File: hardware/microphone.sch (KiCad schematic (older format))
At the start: 9 parts, among them U3 SPH0645LM4H-B

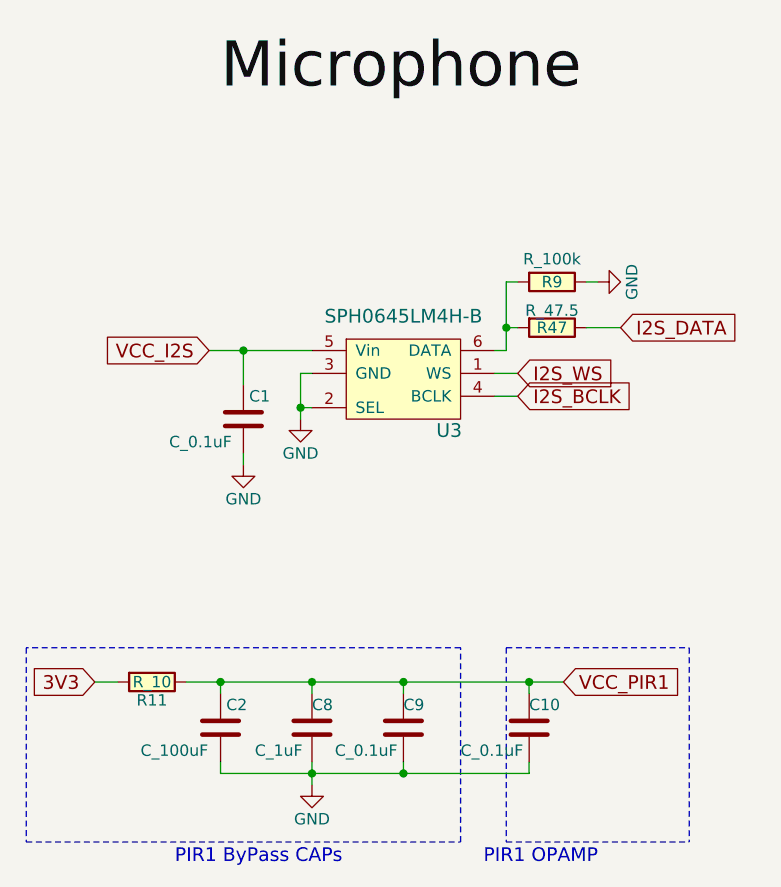
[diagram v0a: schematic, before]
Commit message: update
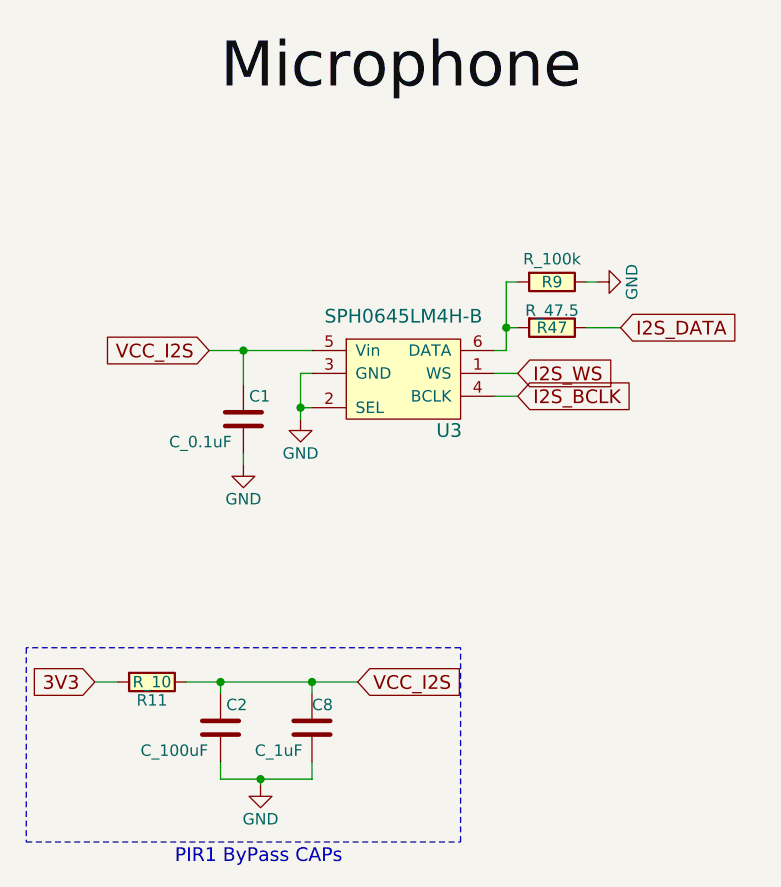
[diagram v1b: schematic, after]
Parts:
- removed C10, C9: C_0.1uF, Capacitors_SMD:C_0603, symbol C_0.1uF
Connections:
- net VCC_PIR1 is gone; now on net VCC_I2S: C2.1, C8.1, R11.1
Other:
- note removed: "PIR1 OPAMP"
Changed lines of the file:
@@
 $EndComp
 $Comp
-L GND #PWR04
+L GND #PWR08
 U 1 1 59AB3AE9
 P 4850 2350
-F 0 "#PWR04" H 4850 2100 50  0001 C CNN
+F 0 "#PWR08" H 4850 2100 50  0001 C CNN
 F 1 "GND" H 4850 2200 50  0000 C CNN
 F 2 "" H 4850 2350 50  0000 C CNN
@@
 	1    0    0    -1
 $EndComp
-Text GLabel 4450 2050 0    60   Input ~ 0
-VCC_I2S
 Text GLabel 5800 2250 2    60   Input ~ 0
 I2S_BCLK
 Text GLabel 6250 1950 2    60   Input ~ 0
 I2S_DATA
-Wire Wire Line
-	5700 2250 5800 2250
-Wire Wire Line
-	5800 2150 5700 2150
-Wire Wire Line
-	4900 2300 4850 2300
-Wire Wire Line
-	4850 2150 4850 2350
-Wire Wire Line
-	4900 2150 4850 2150
-Connection ~ 4850 2300
 Text GLabel 5800 2150 2    60   Input ~ 0
 I2S_WS
-Wire Wire Line
-	4450 2050 4900 2050
 $Comp
 L C_0.1uF C1
@@
 	1    0    0    -1
 $EndComp
-Wire Wire Line
-	4600 2200 4600 2050
-Connection ~ 4600 2050
 $Comp
-L GND #PWR05
+L GND #PWR09
 U 1 1 59B9AD4C
 P 4600 2550
-F 0 "#PWR05" H 4600 2300 50  0001 C CNN
+F 0 "#PWR09" H 4600 2300 50  0001 C CNN
 F 1 "GND" H 4600 2400 50  0000 C CNN
 F 2 "" H 4600 2550 50  0000 C CNN
@@
 	1    0    0    -1
 $EndComp
-Wire Wire Line
-	4600 2500 4600 2550
-Wire Wire Line
-	6100 1950 6250 1950
-Text GLabel 6000 3500 2    60   Input ~ 0
-VCC_PIR1
 $Comp
 L R_10 R11
@@
 $EndComp
 $Comp
-L C_0.1uF C9
-U 1 1 59B80155
-P 5300 3700
-F 0 "C9" H 5300 3800 50  0000 L CNN
-F 1 "C_0.1uF" H 5000 3600 50  0000 L CNN
-F 2 "Capacitors_SMD:C_0603" H 5400 4000 50  0001 C CNN
-F 3 "https://www.digikey.com/product-detail/en/kemet/C0603C104K5RACTU/399-5089-1-ND/1465623" H 5300 3450 50  0001 C CNN
-F 4 "C0603C104K5RACTU" H 5425 3900 60  0001 C CNN "Part Number"
-	1    5300 3700
-	1    0    0    -1
-$EndComp
-$Comp
 L C_100uF C2
 U 1 1 59B80156
@@
 $EndComp
 $Comp
-L GND #PWR06
+L GND #PWR010
 U 1 1 59B80157
-P 4900 3950
-F 0 "#PWR06" H 4900 3700 50  0001 C CNN
-F 1 "GND" H 4900 3800 50  0000 C CNN
-F 2 "" H 4900 3950 50  0000 C CNN
-F 3 "" H 4900 3950 50  0000 C CNN
-	1    4900 3950
+P 4675 3950
+F 0 "#PWR010" H 4675 3700 50  0001 C CNN
+F 1 "GND" H 4675 3800 50  0000 C CNN
+F 2 "" H 4675 3950 50  0000 C CNN
+F 3 "" H 4675 3950 50  0000 C CNN
+	1    4675 3950
 	1    0    0    -1
 $EndComp
 Text GLabel 3950 3500 0    60   Input ~ 0
 3V3
-$Comp
-L C_0.1uF C10
-U 1 1 59B80158
-P 5850 3700
-F 0 "C10" H 5850 3800 50  0000 L CNN
-F 1 "C_0.1uF" H 5550 3600 50  0000 L CNN
-F 2 "Capacitors_SMD:C_0603" H 5950 4000 50  0001 C CNN
-F 3 "https://www.digikey.com/product-detail/en/kemet/C0603C104K5RACTU/399-5089-1-ND/1465623" H 5850 3450 50  0001 C CNN
-F 4 "C0603C104K5RACTU" H 5975 3900 60  0001 C CNN "Part Number"
-	1    5850 3700
-	1    0    0    -1
-$EndComp
 Text Notes 4300 4300 0    60   ~ 0
 PIR1 ByPass CAPs
-Text Notes 5650 4300 0    60   ~ 0
-PIR1 OPAMP
-Wire Wire Line
-	4500 3850 4500 3900
-Wire Wire Line
-	4500 3900 5850 3900
-Wire Wire Line
-	5300 3900 5300 3850
-Wire Wire Line
-	4900 3850 4900 3950
-Connection ~ 4900 3900
-Wire Wire Line
-	4350 3500 6000 3500
-Wire Wire Line
-	5300 3550 5300 3500
-Connection ~ 5300 3500
-Wire Wire Line
-	4900 3550 4900 3500
-Connection ~ 4900 3500
-Wire Wire Line
-	4500 3550 4500 3500
-Connection ~ 4500 3500
-Wire Wire Line
-	3950 3500 4050 3500
-Wire Wire Line
-	5850 3550 5850 3500
-Connection ~ 5850 3500
-Wire Wire Line
-	5850 3900 5850 3850
-Connection ~ 5300 3900
-Wire Notes Line
-	3650 4200 5550 4200
-Wire Notes Line
-	5550 4200 5550 3350
-Wire Notes Line
-	5550 3350 3650 3350
-Wire Notes Line
-	5750 3350 5750 4200
-Wire Notes Line
-	5750 4200 6550 4200
-Wire Notes Line
-	5750 3350 6550 3350
-Wire Notes Line
-	3650 3350 3650 4200
-Wire Notes Line
-	6550 3350 6550 4200
 $Comp
 L R_47.5 R47
@@
 $EndComp
 $Comp
-L GND #PWR07
+L GND #PWR011
 U 1 1 59B820C6
 P 6150 1750
-F 0 "#PWR07" H 6150 1500 50  0001 C CNN
+F 0 "#PWR011" H 6150 1500 50  0001 C CNN
 F 1 "GND" H 6150 1600 50  0000 C CNN
 F 2 "" H 6150 1750 50  0000 C CNN
@@
 	0    -1   -1   0
 $EndComp
+Text GLabel 4450 2050 0    60   Input ~ 0
+VCC_I2S
+Text GLabel 5100 3500 2    60   Input ~ 0
+VCC_I2S
+Connection ~ 4675 3925
 Wire Wire Line
-	6100 1750 6150 1750
+	4675 3950 4675 3925
+Wire Wire Line
+	4900 3925 4500 3925
+Wire Wire Line
+	4900 3850 4900 3925
+Wire Wire Line
+	4350 3500 5100 3500
+Connection ~ 5750 1950
+Wire Wire Line
+	5800 1750 5750 1750
+Wire Wire Line
+	5750 1950 5800 1950
+Wire Wire Line
+	5750 1750 5750 2050
 Wire Wire Line
 	5750 2050 5700 2050
 Wire Wire Line
-	5750 1750 5750 2050
+	6100 1750 6150 1750
+Wire Notes Line
+	3650 3350 3650 4200
+Wire Notes Line
+	5550 3350 3650 3350
+Wire Notes Line
+	5550 4200 5550 3350
+Wire Notes Line
+	3650 4200 5550 4200
 Wire Wire Line
-	5750 1950 5800 1950
+	3950 3500 4050 3500
+Connection ~ 4500 3500
 Wire Wire Line
-	5800 1750 5750 1750
-Connection ~ 5750 1950
+	4500 3550 4500 3500
+Connection ~ 4900 3500
+Wire Wire Line
+	4900 3550 4900 3500
+Wire Wire Line
+	4500 3925 4500 3850
+Wire Wire Line
+	6100 1950 6250 1950
+Wire Wire Line
+	4600 2500 4600 2550
+Connection ~ 4600 2050
+Wire Wire Line
+	4600 2200 4600 2050
+Wire Wire Line
+	4450 2050 4900 2050
+Connection ~ 4850 2300
+Wire Wire Line
+	4900 2150 4850 2150
+Wire Wire Line
+	4850 2150 4850 2350
+Wire Wire Line
+	4900 2300 4850 2300
+Wire Wire Line
+	5800 2150 5700 2150
+Wire Wire Line
+	5700 2250 5800 2250
 $EndSCHEMATC
